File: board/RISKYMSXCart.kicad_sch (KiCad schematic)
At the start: 36 parts, among them CN1 MSX_CART, IC8 LM1117MPX-3.3, J1 Conn_01x02, J2 Conn_01x02, J7 USB_1, J8 Conn_01x02, U1 CH32V307VCT6, U2 MCP6001-OT

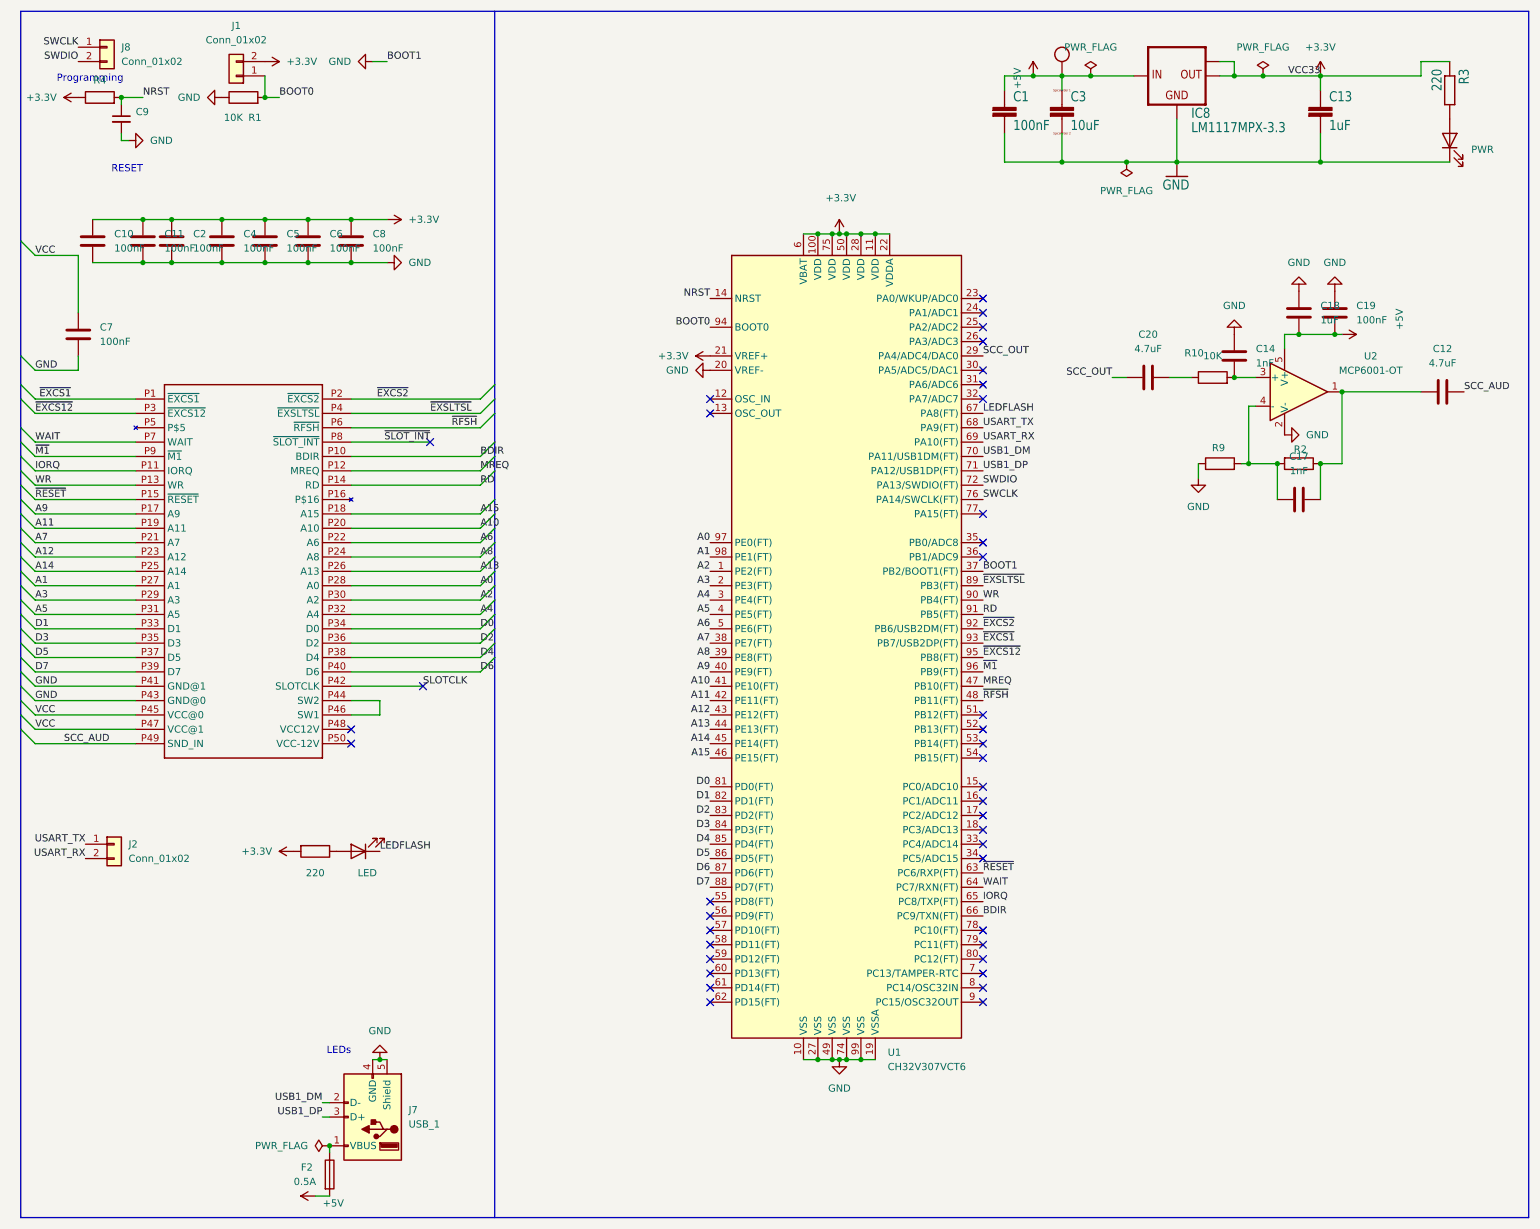
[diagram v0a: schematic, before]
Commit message: New PCB v2.2
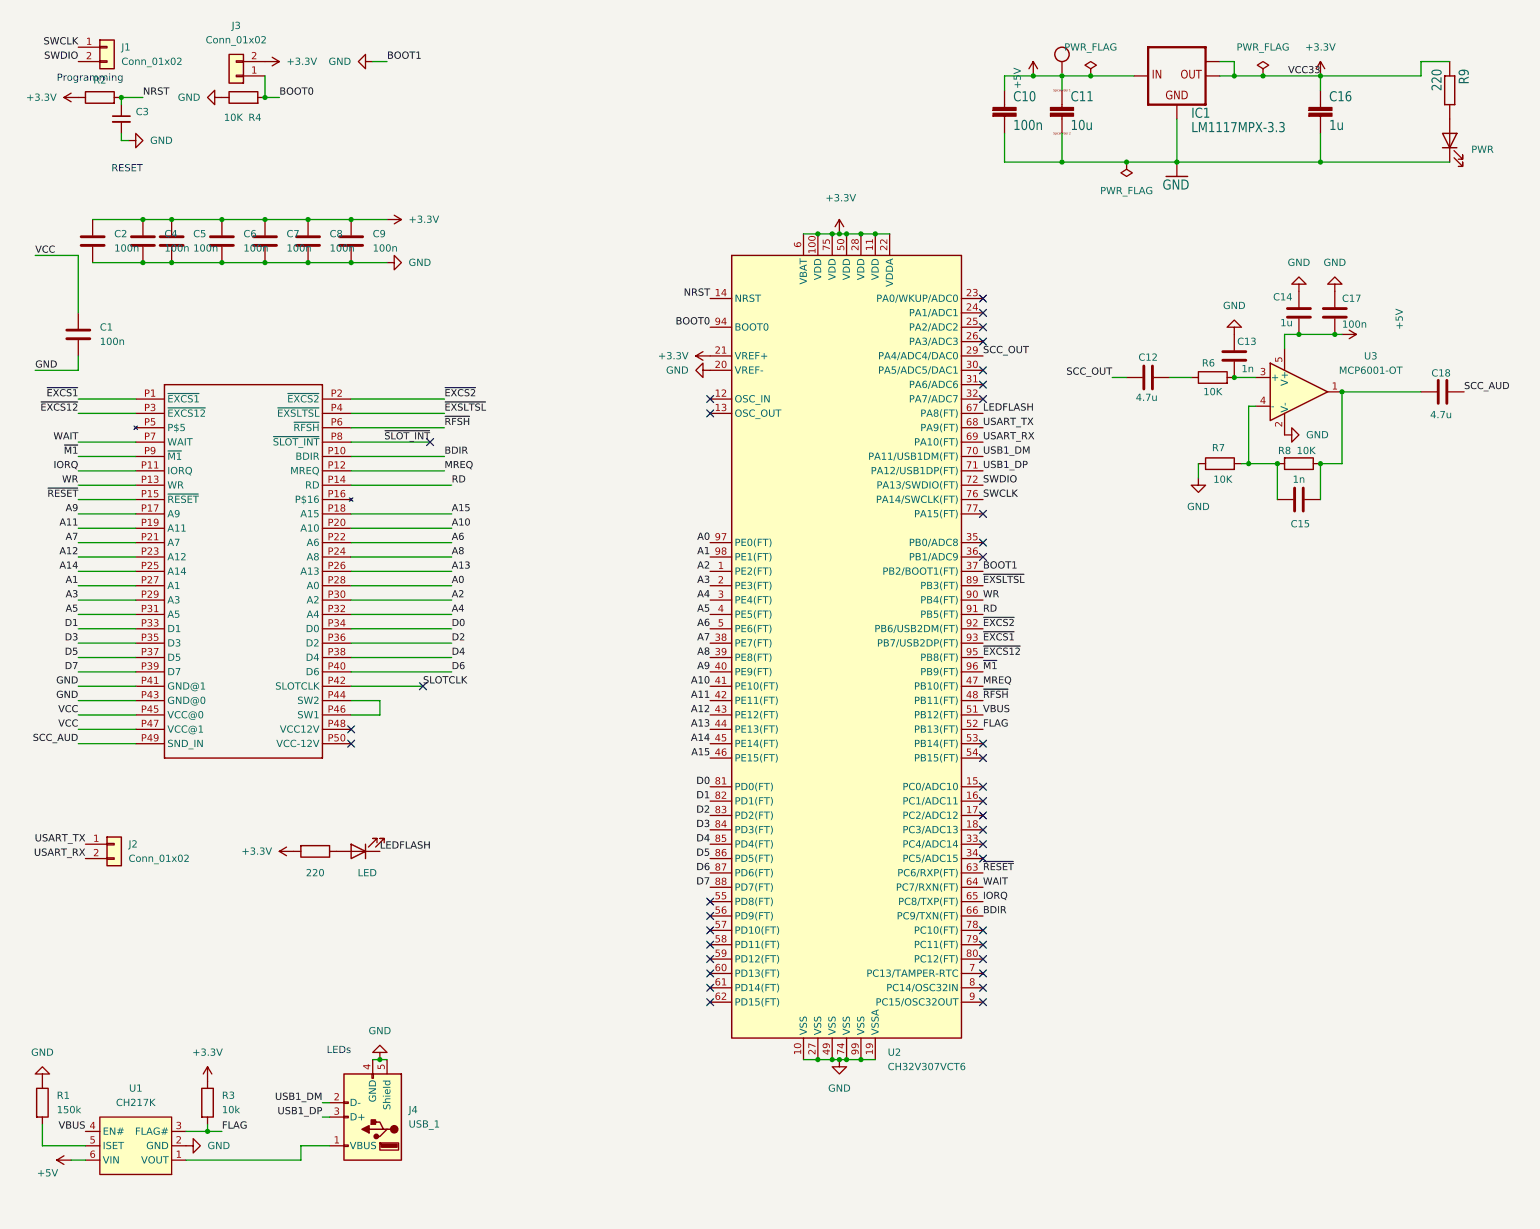
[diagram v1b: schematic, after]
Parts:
- removed F2: 0.5A, Fuse:Fuse_1206_3216Metric_Pad1.42x1.75mm_HandSolder, symbol Device:Fuse
- added R1: 150k, Resistor_SMD:R_0603_1608Metric_Pad0.98x0.95mm_HandSolder, symbol Device:R
- added R3: 10k, Resistor_SMD:R_0603_1608Metric_Pad0.98x0.95mm_HandSolder, symbol Device:R
- added U1: CH217K, Package_TO_SOT_SMD:SOT-23-6, symbol wch_mcu_peripheral:CH217K
- C1: renamed from C7; value 100nF -> 100n
- C10: renamed from C1; value 100nF -> 100n
- C11: renamed from C3; value 10uF -> 10u
- C12: renamed from C20; value 4.7uF -> 4.7u
- C13: renamed from C14; value 1nF -> 1n
- C14: renamed from C18; value 1uF -> 1u
- C15: renamed from C17; value 1nF -> 1n
- C16: renamed from C13; value 1uF -> 1u
- C17: renamed from C19; value 100nF -> 100n
- C18: renamed from C12; value 4.7uF -> 4.7u
- C2: renamed from C10; value 100nF -> 100n
- C3: renamed from C9; value 100nF -> 100n
- C4: renamed from C11; value 100nF -> 100n
- C5: renamed from C2; value 100nF -> 100n
- C6: renamed from C4; value 100nF -> 100n
- C7: renamed from C5; value 100nF -> 100n
- C8: renamed from C6; value 100nF -> 100n
- C9: renamed from C8; value 100nF -> 100n
- renumbered D5 to D2, IC8 to IC1, J8 to J1, J1 to J3, J7 to J4, R4 to R2, R1 to R4, R10 to R6, R9 to R7, R2 to R8, R3 to R9, U1 to U2, U2 to U3
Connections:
- net +3.3V: now also R3.1
- net +5V: now also U1.6 (VIN)
- net GND: now also R1.1, U1.2 (GND)
- net at J4.1 (VBUS): now also U1.1 (VOUT)
- net VBUS: now reaches U2.51 (PB12(FT))
- net VBUS: now also U1.4 (EN#)
- net FLAG: now reaches U2.52 (PB13(FT))
- net FLAG: now also R3.2, U1.3 (FLAG#)
- new net: R1.2, U1.5 (ISET)
- no-connect marks 40 -> 38
